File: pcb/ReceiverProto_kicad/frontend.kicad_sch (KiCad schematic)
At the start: 30 parts, among them Q1 Q_NPN_BCE, Q2 NJFET, Q3 NJFET, U1 AD8001AN

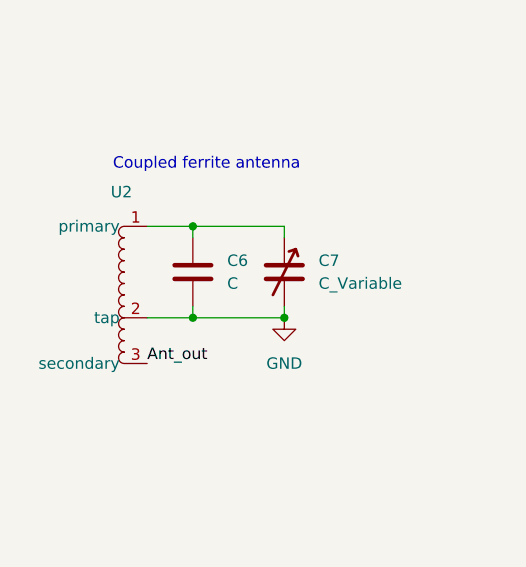
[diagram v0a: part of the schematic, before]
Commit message: finished moving over project to this repo
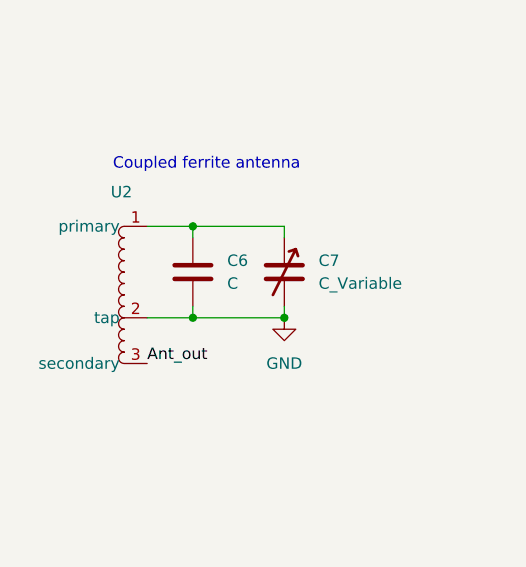
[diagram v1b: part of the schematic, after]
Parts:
- removed U2: ~, symbol custom_lib:Ferrite_Antenna_tapped
- added U2: ~, symbol antenna:Ferrite_antenna_tapped
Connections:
- net GND: now also U2.2 (tap)
- net SIM_Vin: now also U2.3 (secondary)
- net at C6.1, C7.1: now also U2.1 (primary)
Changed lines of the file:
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@@
 			)
 		)
-		(property "Sim.Library" "/home/aidan/KiCad-Spice-Library/Models/uncategorized/spice_complete/AD6A.LIB"
+		(property "Sim.Library" "../spice_libraries/KiCad-Spice-Library/Models/uncategorized/spice_complete/AD6A.LIB"
 			(at 116.84 128.27 0)
 			(effects
@@
 	)
 	(symbol
+		(lib_id "antenna:Ferrite_antenna_tapped")
+		(at 41.91 69.85 0)
+		(unit 1)
+		(exclude_from_sim yes)
+		(in_bom yes)
+		(on_board yes)
+		(dnp no)
+		(fields_autoplaced yes)
+		(property "Reference" "U2"
+			(at 39.0525 68.58 0)
+			(effects
+				(font
+					(size 1.27 1.27)
+				)
+			)
+		)
+		(property "Value" "~"
+			(at 39.0525 71.12 0)
+			(effects
+				(font
+					(size 1.27 1.27)
+				)
+			)
+		)
+		(property "Footprint" ""
+			(at 41.91 69.85 0)
+			(effects
+				(font
+					(size 1.27 1.27)
+				)
+				(hide yes)
+			)
+		)
+		(property "Datasheet" ""
+			(at 41.91 69.85 0)
+			(effects
+				(font
+					(size 1.27 1.27)
+				)
+				(hide yes)
+			)
+		)
+		(property "Description" ""
+			(at 41.91 69.85 0)
+			(effects
+				(font
+					(size 1.27 1.27)
+				)
+				(hide yes)
+			)
+		)
+		(pin "2"
+		)
+		(pin "1"
+		)
+		(pin "3"
+		)
+		(instances
+			(project ""
+				(path "/1f346c8c-1e51-4f75-85ee-2d30c45e3fc5/91368719-672a-4a05-ad25-dcc79ecf4ba6"
+					(reference "U2")
+					(unit 1)
+				)
+			)
+		)
+	)
+	(symbol
 		(lib_id "power:GND")
 		(at 57.15 82.55 0)
@@
 	)
 	(symbol
-		(lib_id "custom_lib:Ferrite_Antenna_tapped")
-		(at 39.37 69.85 0)
-		(unit 1)
-		(exclude_from_sim yes)
-		(in_bom yes)
-		(on_board yes)
-		(dnp no)
-		(fields_autoplaced yes)
-		(property "Reference" "U2"
-			(at 39.0525 68.58 0)
-			(effects
-				(font
-					(size 1.27 1.27)
-				)
-			)
-		)
-		(property "Value" "~"
-			(at 39.0525 71.12 0)
-			(effects
-				(font
-					(size 1.27 1.27)
-				)
-			)
-		)
-		(property "Footprint" ""
-			(at 39.37 69.85 0)
-			(effects
-				(font
-					(size 1.27 1.27)
-				)
-				(hide yes)
-			)
-		)
-		(property "Datasheet" ""
-			(at 39.37 69.85 0)
-			(effects
-				(font
-					(size 1.27 1.27)
-				)
-				(hide yes)
-			)
-		)
-		(property "Description" ""
-			(at 39.37 69.85 0)
-			(effects
-				(font
-					(size 1.27 1.27)
-				)
-				(hide yes)
-			)
-		)
-		(pin "2"
-		)
-		(pin "1"
-		)
-		(pin "3"
-		)
-		(instances
-			(project "ReceiverProto"
-				(path "/1f346c8c-1e51-4f75-85ee-2d30c45e3fc5/91368719-672a-4a05-ad25-dcc79ecf4ba6"
-					(reference "U2")
-					(unit 1)
-				)
-			)
-		)
-	)
-	(symbol
 		(lib_id "Device:R")
 		(at 140.97 80.01 0)
@@
 			)
 		)
-		(property "Sim.Library" "spice/2N3904"
+		(property "Sim.Library" "/home/aidan/Avy-Dawgs/pcb/spice_libraries/misc/2N3904"
 			(at 138.43 68.58 0)
 			(effects
